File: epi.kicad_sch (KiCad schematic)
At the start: 31 parts, among them J1 Connector 1x12, J2 Connector 1x12, J3 Conn_01x05, J4 USB-C 2.0 mid-mount female co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, U1 ATmega32U4-M, Y1 Crystal_GND24

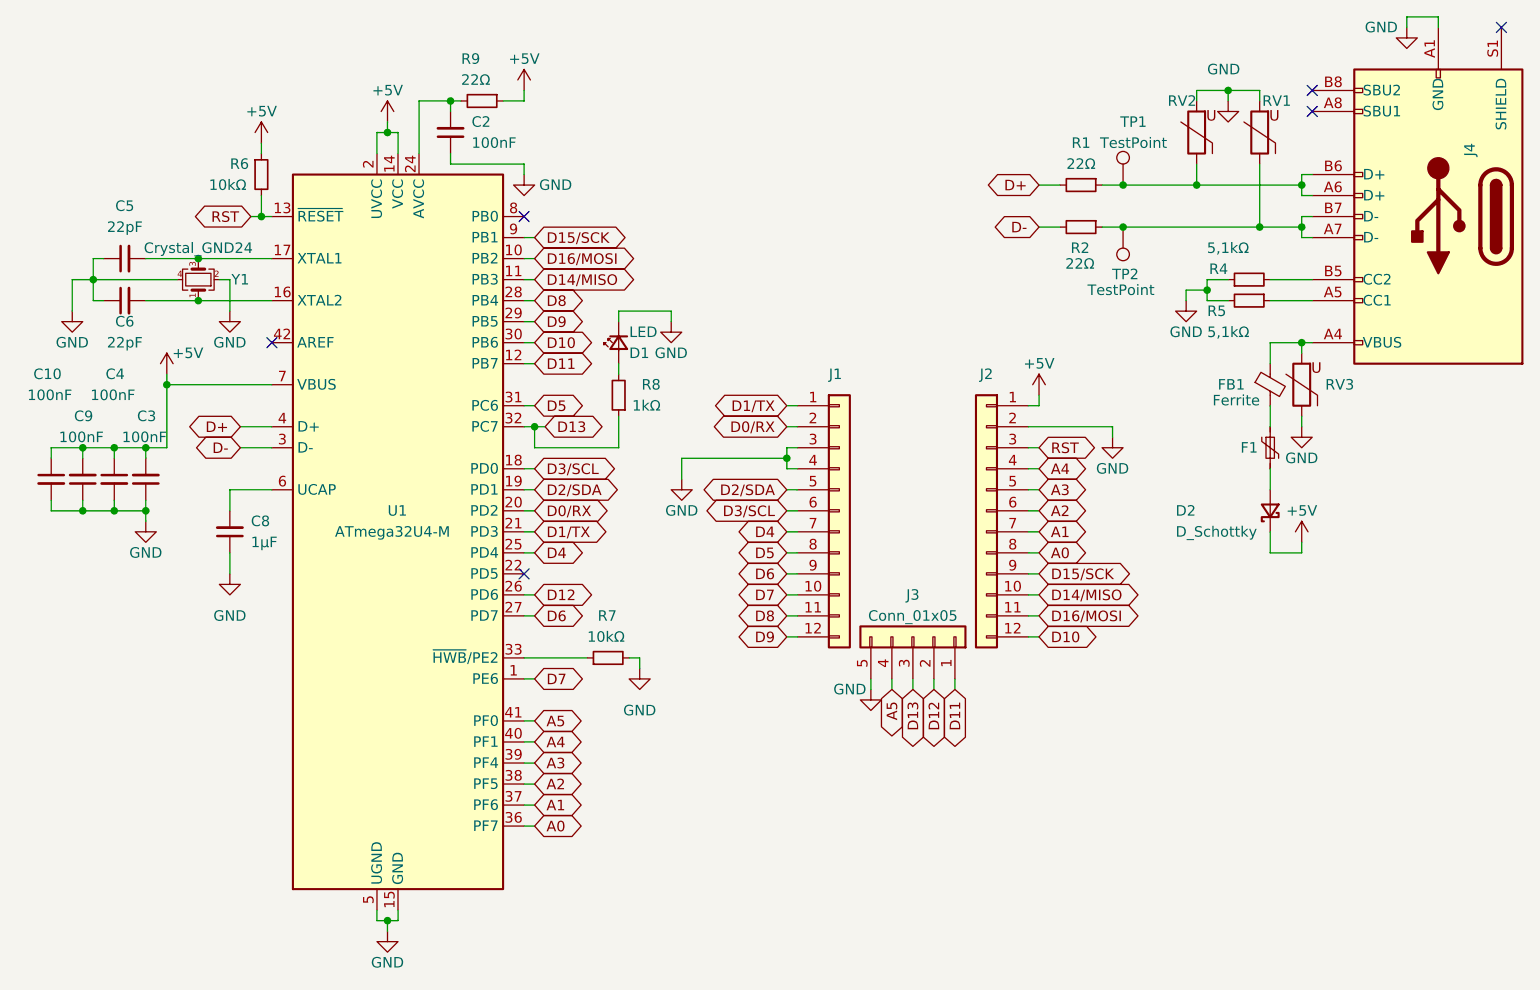
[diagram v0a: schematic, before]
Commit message: new computer, new updates
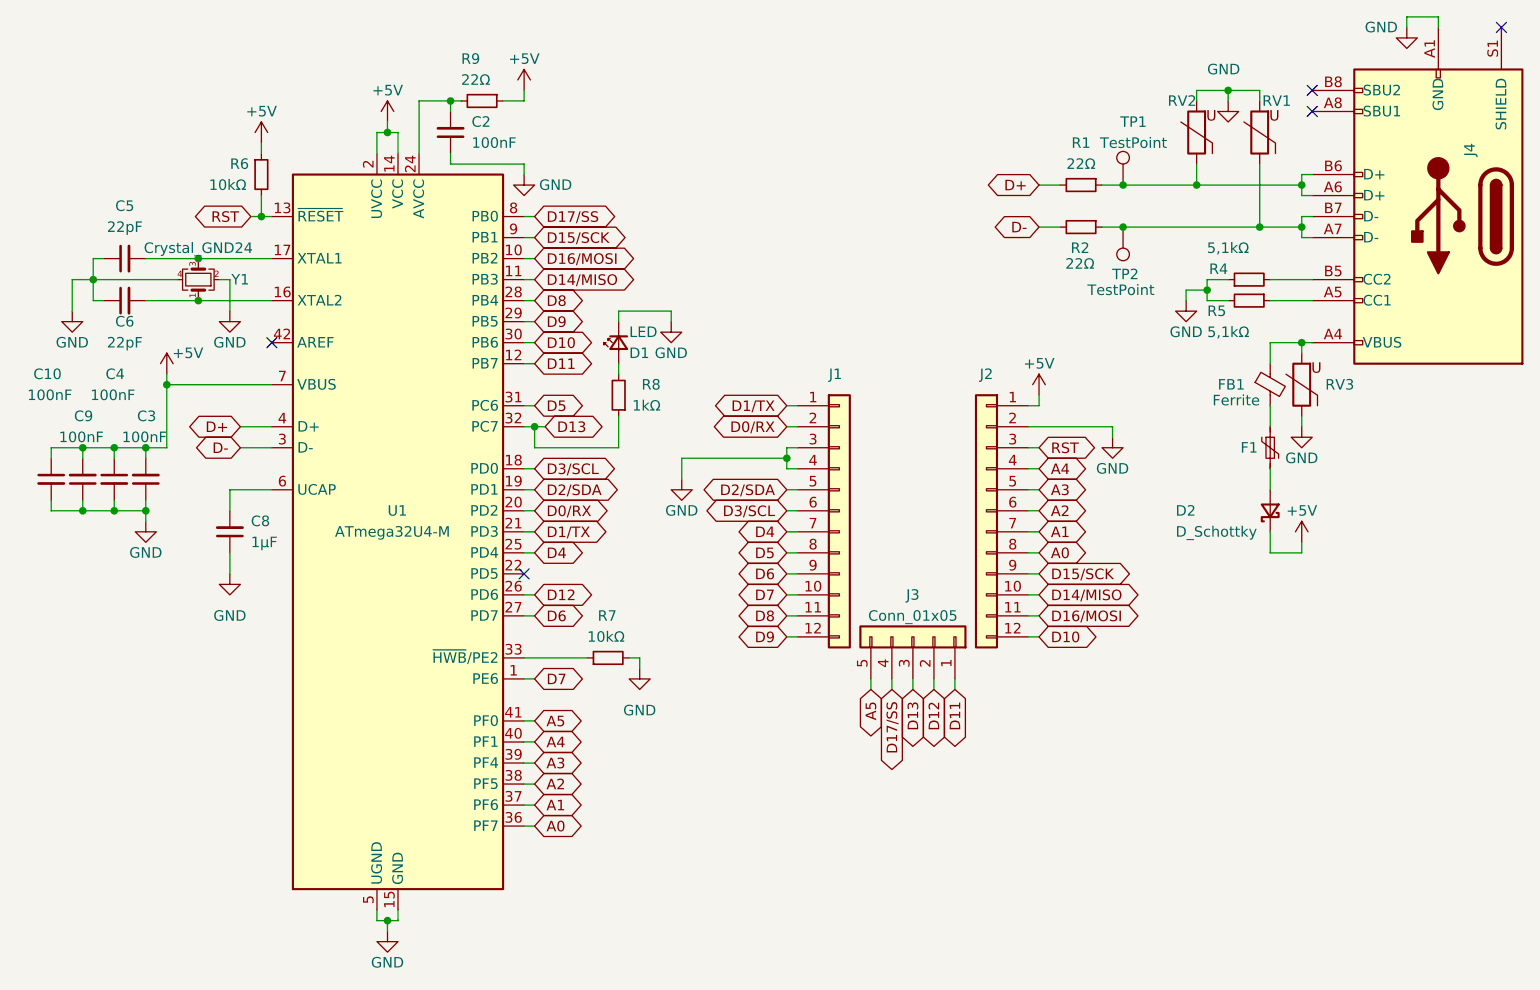
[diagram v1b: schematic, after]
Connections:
- net A5: now also J3.5 (Pin_5); no longer J3.4 (Pin_4)
- net GND: no longer J3.5 (Pin_5)
- net D17/SS: now reaches U1.8 (PB0)
- net D17/SS: now also J3.4 (Pin_4)
- no-connect marks 6 -> 5
